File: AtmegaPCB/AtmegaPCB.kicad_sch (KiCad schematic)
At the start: 175 parts, among them SW1 SW_Push, U1 PRTR5V0U2X, U2 ATmega32U4-A, Y1 16MHz

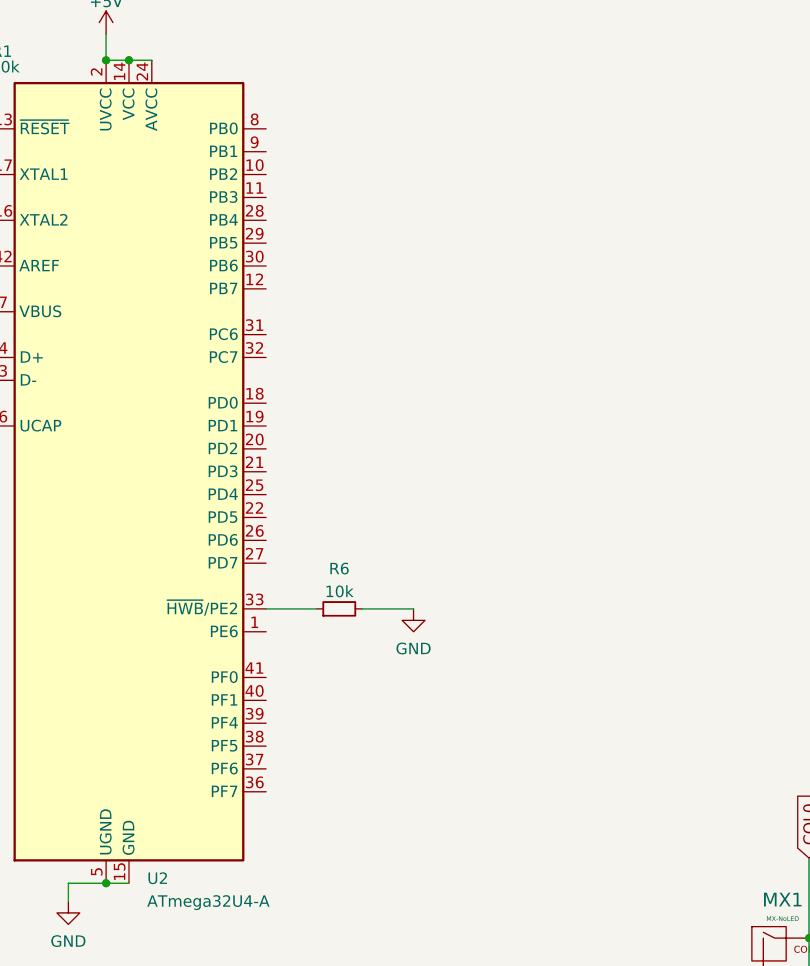
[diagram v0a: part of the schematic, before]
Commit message: COL & ROW Traced
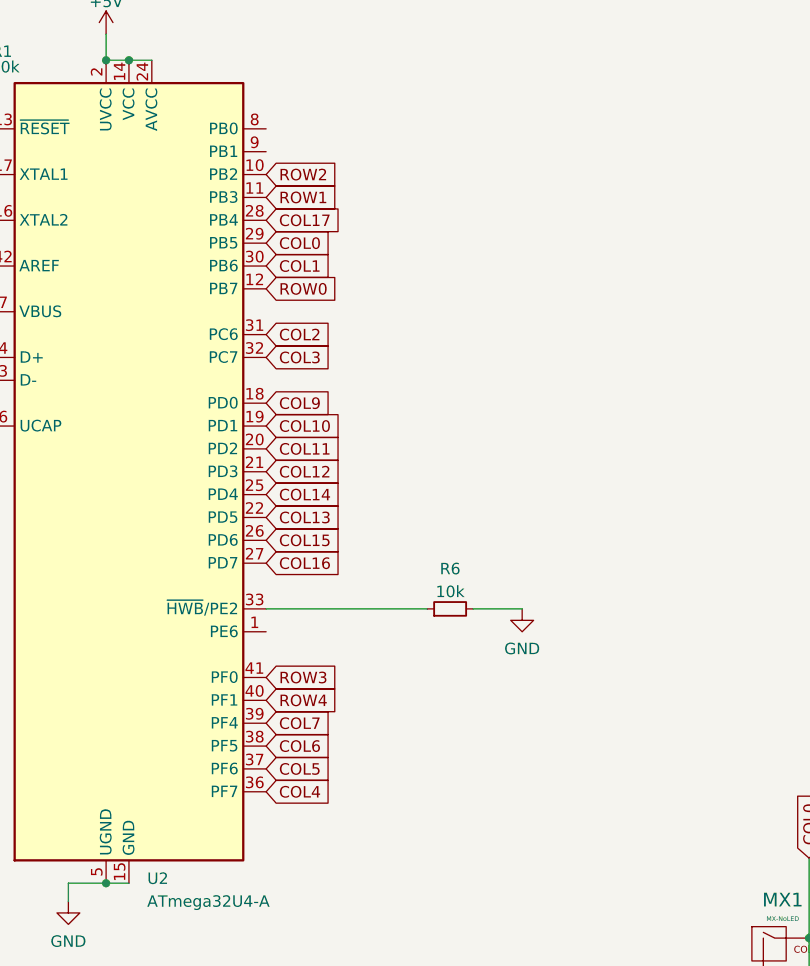
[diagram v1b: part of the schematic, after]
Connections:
- net COL0: now also U2.29 (PB5)
- net COL1: now also U2.30 (PB6)
- net COL10: now also U2.19 (PD1)
- net COL11: now also U2.20 (PD2)
- net COL12: now also U2.21 (PD3)
- net COL13: now also U2.22 (PD5)
- net COL14: now also U2.25 (PD4)
- net COL15: now also U2.26 (PD6)
- net COL16: now also U2.27 (PD7)
- net COL17: now also U2.28 (PB4)
- net COL2: now also U2.31 (PC6)
- net COL3: now also U2.32 (PC7)
- net COL4: now also U2.36 (PF7)
- net COL5: now also U2.37 (PF6)
- net COL6: now also U2.38 (PF5)
- net COL7: now also U2.39 (PF4)
- net COL9: now also U2.18 (PD0)
- net ROW0: now also U2.12 (PB7)
- net ROW1: now also U2.11 (PB3)
- net ROW2: now also U2.10 (PB2)
- net ROW3: now also U2.41 (PF0)
- net ROW4: now also U2.40 (PF1)
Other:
- moved on the sheet: R6
